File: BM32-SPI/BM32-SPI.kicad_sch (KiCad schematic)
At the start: 12 parts, among them U1 XC6209F332MR, U2 W25Q32JVSS

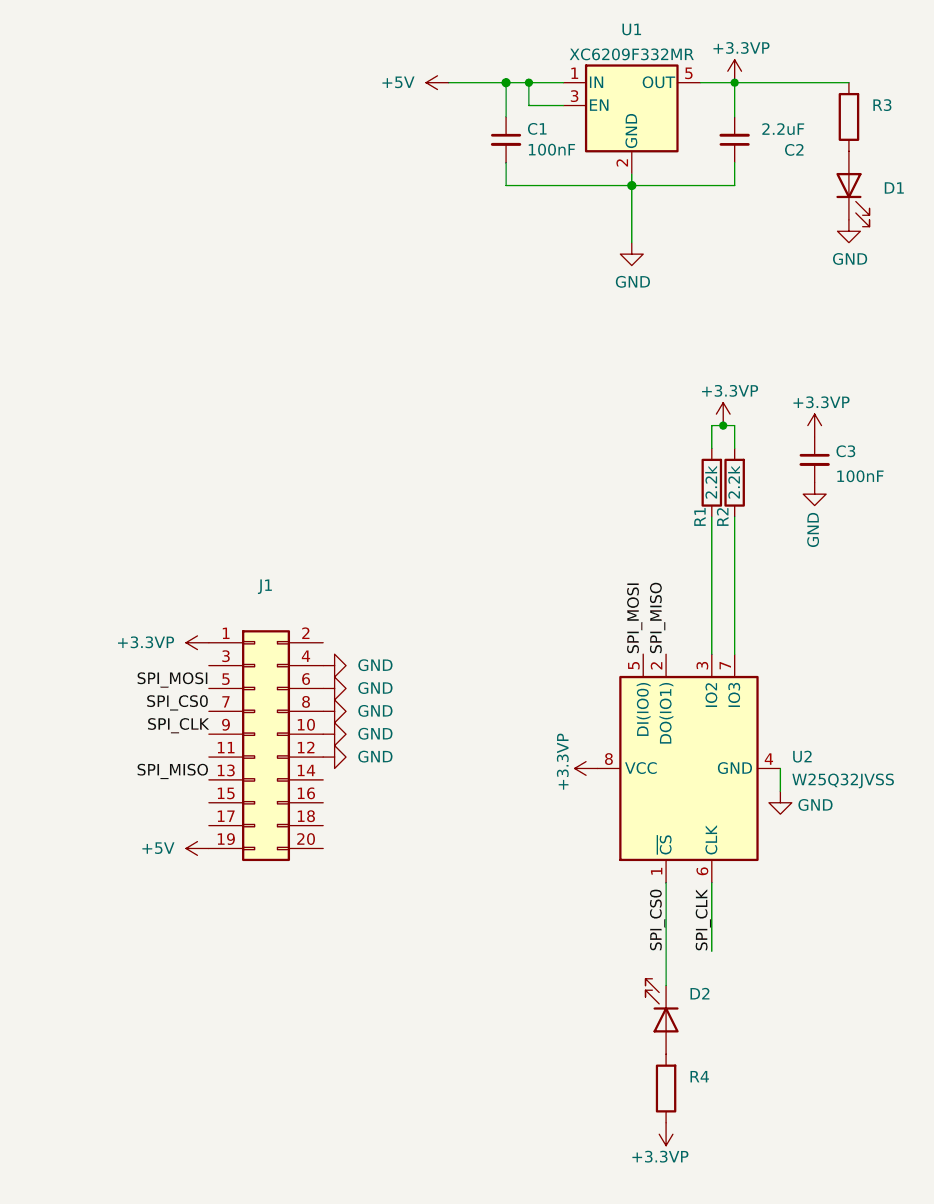
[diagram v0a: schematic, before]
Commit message: Update
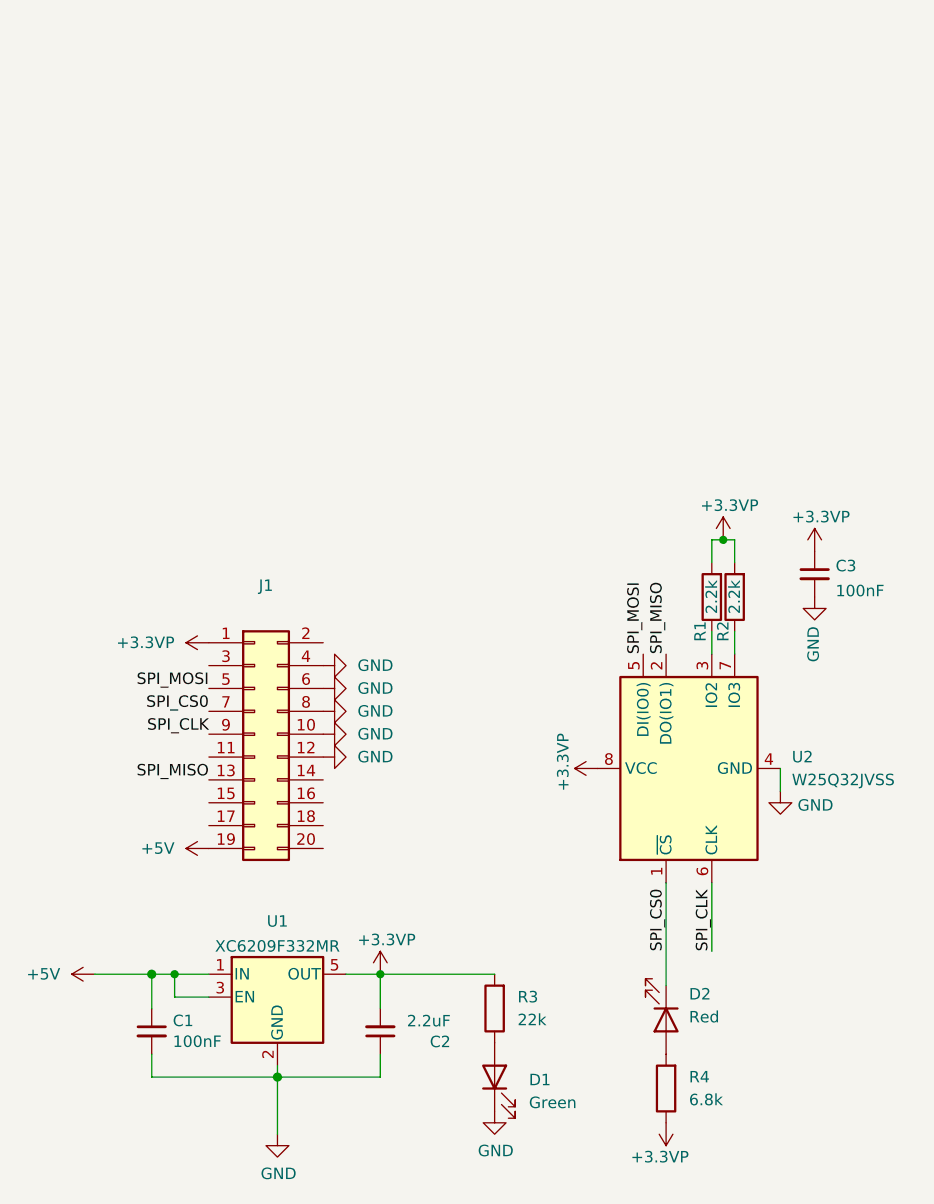
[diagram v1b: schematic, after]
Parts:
- D1: value (none) -> Green; footprint (none) -> lc:0805_LED_S1_NUM
- D2: value (none) -> Red
- R3: value (none) -> 22k; footprint (none) -> lc:0402_R
- R4: value (none) -> 6.8k
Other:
- moved on the sheet: C1, C2, C3, D1, R1, R2, R3, U1
